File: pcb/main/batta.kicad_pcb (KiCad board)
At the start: 2 copper layers, 126.9 x 99.3 mm, 42 parts

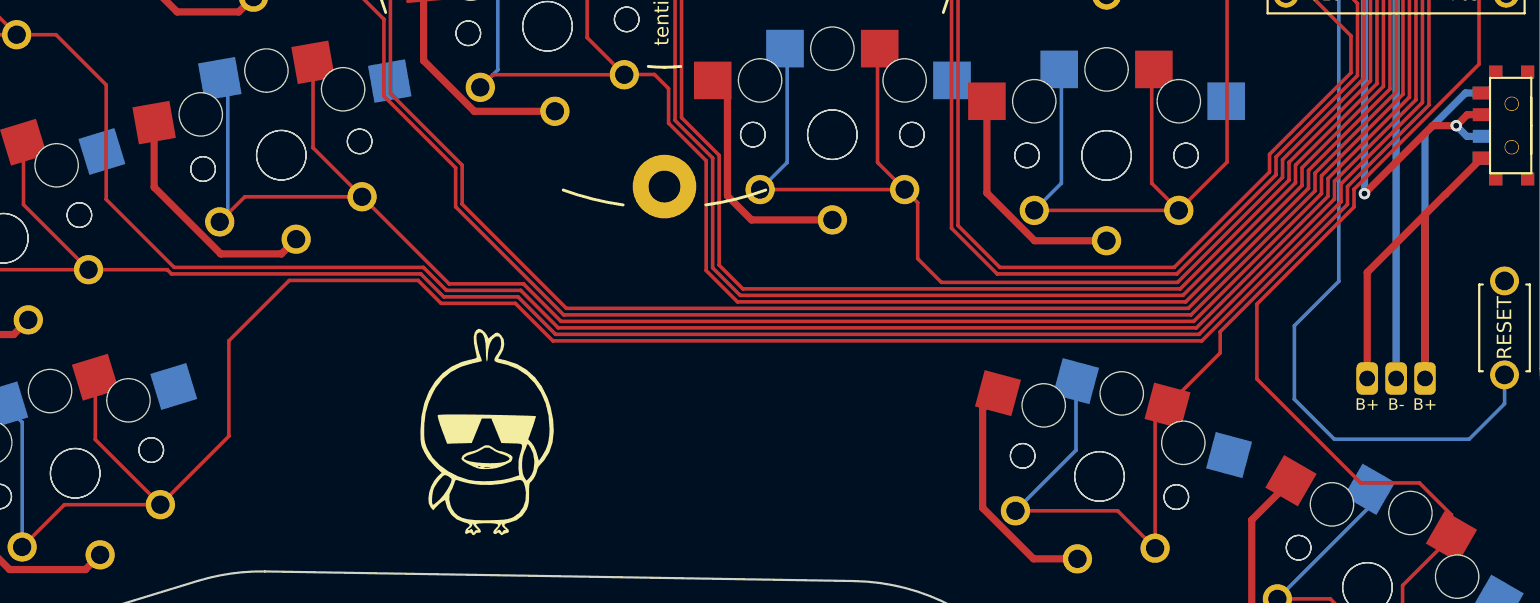
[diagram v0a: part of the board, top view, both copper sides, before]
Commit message: clean router in batta main
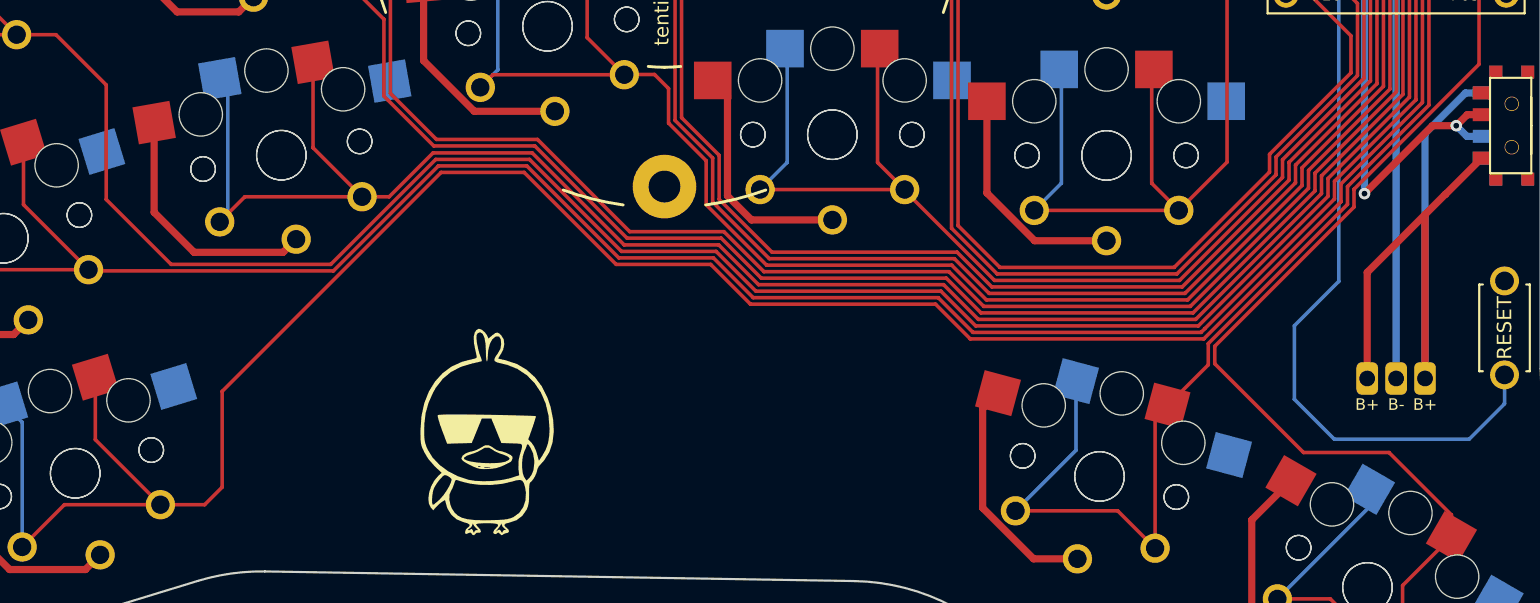
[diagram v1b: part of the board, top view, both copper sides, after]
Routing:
- net P6: track 157.1 -> 163.2 mm
- net P5: track 152.9 -> 158.8 mm
- net P4: track 172.2 -> 178.1 mm
- net P8: track 86.8 -> 90.3 mm
- net P1: track 142.3 -> 139.5 mm
- net P15: track 152.4 -> 149.6 mm
- net P18: track 138.9 -> 136.1 mm
- net P3: track 139.5 -> 141.9 mm
- net P14: track 89.2 -> 86.9 mm
- net P2: track 157.0 -> 155.3 mm
- net P0: track 183.1 -> 181.4 mm
- net GND: track 274.9 -> 275.8 mm

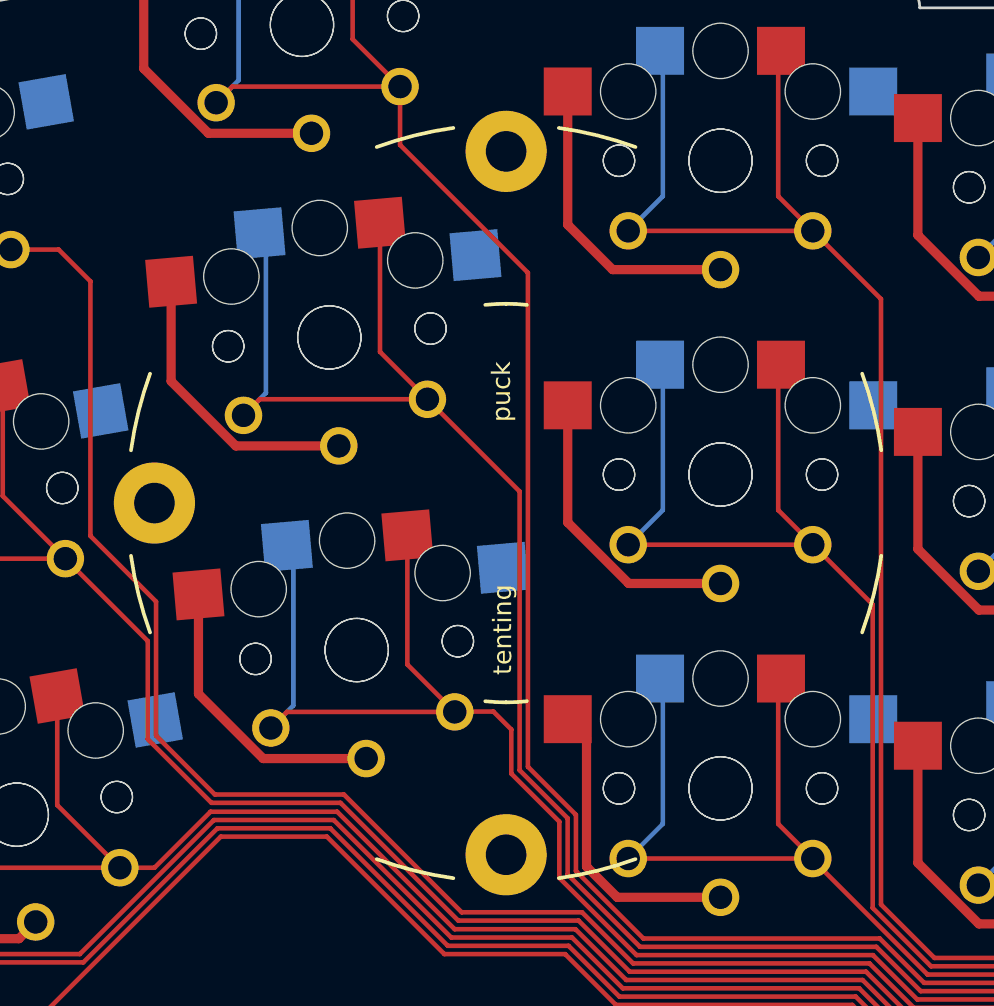
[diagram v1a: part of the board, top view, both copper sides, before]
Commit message: updated gerber
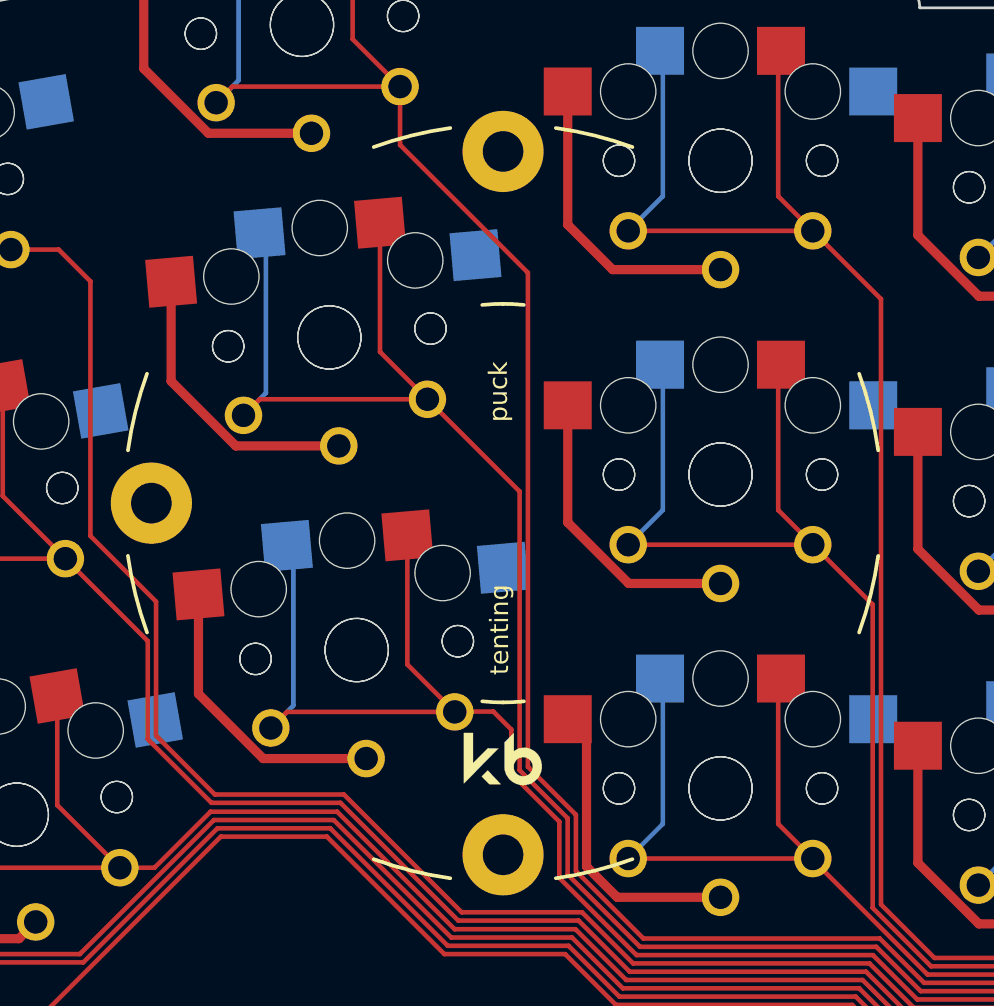
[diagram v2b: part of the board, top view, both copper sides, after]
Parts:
- removed the REF** at (103.8, -88.1)
- added REF**: Tenting Puck, kbd:Tenting_Puck2, F.Cu at (103.6, -88.1)
